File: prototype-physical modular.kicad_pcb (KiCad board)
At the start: 2 copper layers, 100 x 164 mm, 183 parts, among them CON1 BARREL_JACK, CON2 SD_Card_SEEEDOPL, IC1 ATMEGA2560-A, P1 POWER, P10 PC, P11 CONN_UART, P12 PJ, P15 PH, P16 PF, P18 3VI2C, P19 PIGPIO, P20 MIDI_IN, P21 MIDI_OUT, P22 BUSTI, P23 BUSTO, P3 SPI, P7 PA, Q1 BSS138, Q2 BSS138, Q3 BSS138, Q4 BSS138, Q5 BSS138, Q6 BSS138, SW1 SW_PUSH, SW10 SW_PUSH, SW11 SW_PUSH, SW12 SW_PUSH, SW13 SW_PUSH, SW14 SW_PUSH, SW2 ROTARY_ENCODER_SWITCH, SW3 SW_PUSH, SW4 SW_PUSH, SW5 SW_PUSH, SW6 SW_PUSH, SW7 SW_PUSH, SW8 SW_PUSH, SW9 SW_PUSH, U1 NCP1117ST50T3G, U2 6N138, Y1 16MHz

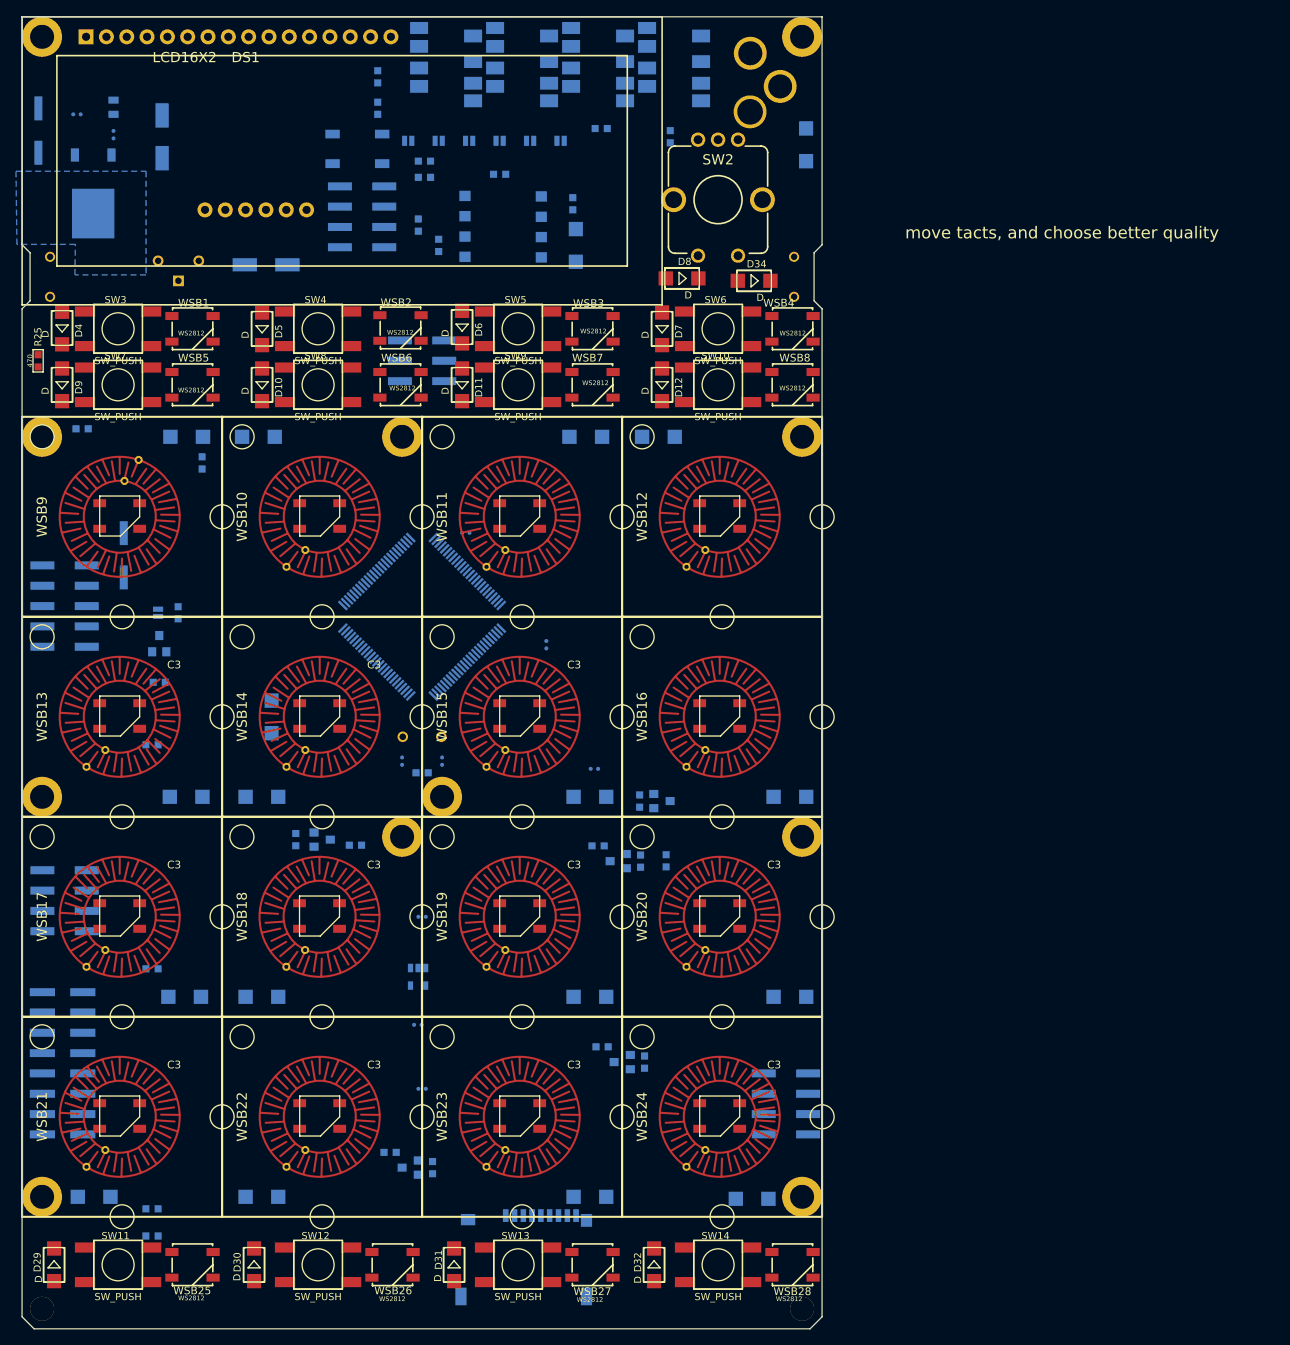
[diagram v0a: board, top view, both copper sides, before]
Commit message: routed
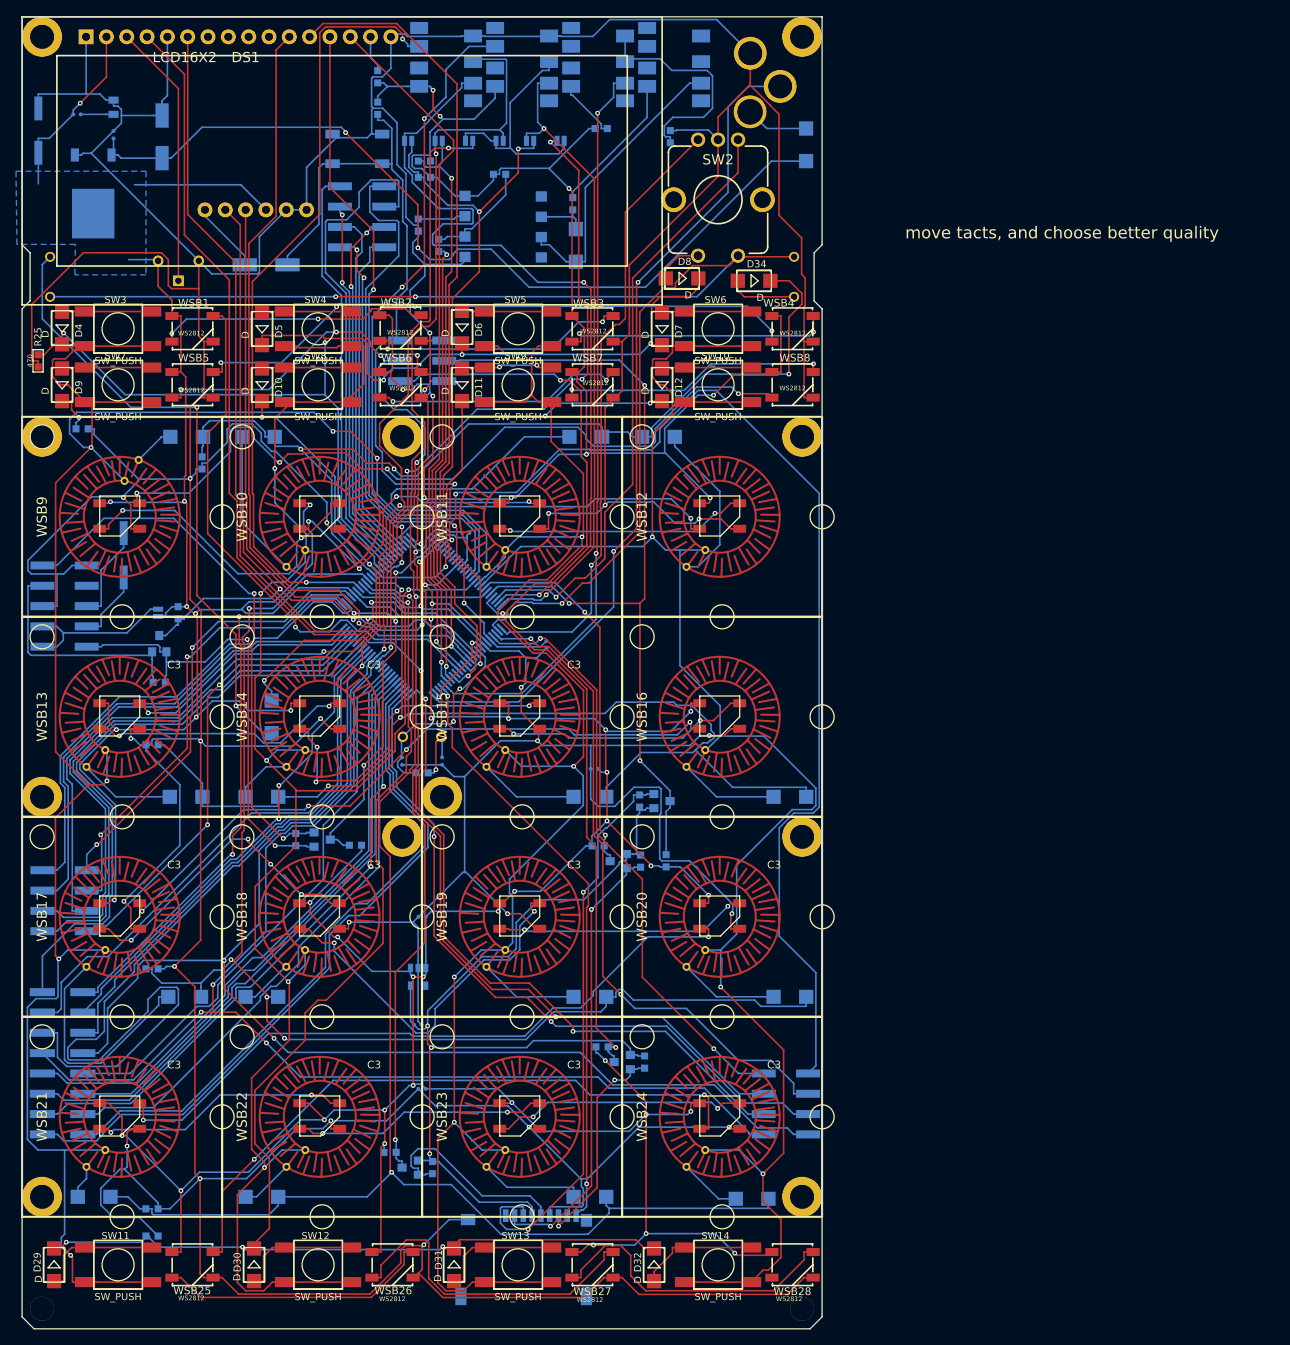
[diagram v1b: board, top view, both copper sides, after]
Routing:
- net GND: track 0.00 -> 1129.8 mm, vias 0 -> 27
- net +5V: track 0.00 -> 814.1 mm, vias 0 -> 51
- net /MUXAX0: track 0.00 -> 257.5 mm, vias 0 -> 6
- net /BUS_COM: track 0.00 -> 250.1 mm, vias 0 -> 5
- net /TX3: track 0.00 -> 241.9 mm, vias 0 -> 6
- net /MUXAX1: track 0.00 -> 228.1 mm, vias 0 -> 6
- net /MUXAX3: track 0.00 -> 215.5 mm, vias 0 -> 3
- net /MUXAX2: track 0.00 -> 204.7 mm, vias 0 -> 4
- net Net-(IC1-Pad65): track 0.00 -> 191.4 mm, vias 0 -> 2
- net /MUXBX6: track 0.00 -> 178.5 mm, vias 0 -> 4
- net /MUXBX5: track 0.00 -> 175.0 mm, vias 0 -> 2
- net /MUXAX4: track 0.00 -> 163.0 mm, vias 0 -> 3
- net /MUXBX4: track 0.00 -> 161.9 mm, vias 0 -> 4
- net /MUXBX0: track 0.00 -> 144.8 mm, vias 0 -> 5
- net Net-(IC1-Pad1): track 0.00 -> 144.5 mm, vias 0 -> 2
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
